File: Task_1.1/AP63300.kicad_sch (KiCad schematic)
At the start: 10 parts, among them J1 Conn_01x03, U1 AP63300

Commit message: Fixed and updated part numbers and pcb schematics
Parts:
- C1: footprint Capacitor_SMD:C_1206_3216Metric -> Capacitor_SMD:C_1210_3225Metric
- C21, C22: footprint Capacitor_SMD:C_0201_0603Metric -> Capacitor_SMD:C_1210_3225Metric
- C3: footprint Capacitor_SMD:C_0201_0603Metric -> Capacitor_SMD:C_0603_1608Metric; MPN GRM033C71C104KE14D -> CC0603KRX7R7BB104
- C4: footprint Capacitor_SMD:C_0201_0603Metric -> Capacitor_SMD:C_0603_1608Metric; MPN GRM0335C1E470FA01D -> 885012006021
- R1: footprint Resistor_SMD:R_0201_0603Metric -> Resistor_SMD:R_0603_1608Metric; MPN ERJ-1GNF1583C -> RC0603FR-07158KL
- R2: footprint Resistor_SMD:R_0201_0603Metric -> Resistor_SMD:R_0603_1608Metric; MPN ERJ-1GNF3012C -> RK73H1JTTD3012F
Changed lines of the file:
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@@
 			)
 		)
-		(property "Footprint" "Resistor_SMD:R_0201_0603Metric"
+		(property "Footprint" "Resistor_SMD:R_0603_1608Metric"
 			(at 99.822 59.69 90)
 			(hide yes)
@@
 			)
 		)
-		(property "Datasheet" "https://industrial.panasonic.com/cdbs/www-data/pdf/RDA0000/AOA0000C304.pdf"
+		(property "Datasheet" "https://www.koaspeer.com/pdfs/RK73H.pdf"
 			(at 101.6 59.69 0)
 			(hide yes)
@@
 			)
 		)
-		(property "Description" "30.1 kOhms ±1% 0.05W, 1/20W Chip Resistor 0201 (0603 Metric) Thick Film"
+		(property "Description" "30.1 kOhms ±1% 0.1W, 1/10W Chip Resistor 0603 (1608 Metric) Automotive AEC-Q200 Thick Film"
 			(at 101.6 59.69 0)
 			(hide yes)
@@
 			)
 		)
-		(property "MPN" "ERJ-1GNF3012C"
+		(property "MPN" "RK73H1JTTD3012F"
 			(at 101.6 59.69 0)
 			(hide yes)
@@
 			)
 		)
-		(property "Footprint" "Capacitor_SMD:C_0201_0603Metric"
+		(property "Footprint" "Capacitor_SMD:C_1210_3225Metric"
 			(at 120.3452 59.69 0)
 			(hide yes)
@@
 			)
 		)
-		(property "Footprint" "Resistor_SMD:R_0201_0603Metric"
+		(property "Footprint" "Resistor_SMD:R_0603_1608Metric"
 			(at 99.822 52.07 90)
 			(hide yes)
@@
 			)
 		)
-		(property "Datasheet" "https://industrial.panasonic.com/cdbs/www-data/pdf/RDA0000/AOA0000C304.pdf"
+		(property "Datasheet" "https://yageogroup.com/content/datasheet/asset/file/PYU-RC_GROUP_51_ROHS_L"
 			(at 101.6 52.07 0)
 			(hide yes)
@@
 			)
 		)
-		(property "Description" "158 kOhms ±1% 0.05W, 1/20W Chip Resistor 0201 (0603 Metric) Thick Film"
+		(property "Description" "158 kOhms ±1% 0.1W, 1/10W Chip Resistor 0603 (1608 Metric) Moisture Resistant Thick Film"
 			(at 101.6 52.07 0)
 			(hide yes)
@@
 			)
 		)
-		(property "MPN" "ERJ-1GNF1583C"
+		(property "MPN" "RC0603FR-07158KL"
 			(at 101.6 52.07 0)
 			(hide yes)
@@
 			)
 		)
-		(property "Footprint" "Capacitor_SMD:C_0201_0603Metric"
+		(property "Footprint" "Capacitor_SMD:C_0603_1608Metric"
 			(at 96.2152 55.88 0)
 			(hide yes)
@@
 			)
 		)
-		(property "Datasheet" "https://mm.digikey.com/Volume0/opasdata/d220001/medias/docus/8942/490_Chip_Multilayer_CAT2021_MLCC.pdf"
+		(property "Datasheet" "https://www.we-online.com/components/products/datasheet/885012006021.pdf"
 			(at 95.25 52.07 0)
 			(hide yes)
@@
 			)
 		)
-		(property "Description" "47 pF ±1% 25V Ceramic Capacitor C0G, NP0 0201 (0603 Metric)"
+		(property "Description" "47 pF ±5% 16V Ceramic Capacitor C0G, NP0 0603 (1608 Metric)"
 			(at 95.25 52.07 0)
 			(hide yes)
@@
 			)
 		)
-		(property "MPN" "GRM0335C1E470FA01D"
+		(property "MPN" "885012006021"
 			(at 95.25 52.07 0)
 			(hide yes)
@@
 			)
 		)
-		(property "Footprint" "Capacitor_SMD:C_1206_3216Metric"
+		(property "Footprint" "Capacitor_SMD:C_1210_3225Metric"
 			(at 39.0652 57.15 0)
 			(hide yes)
@@
 			)
 		)
-		(property "Footprint" "Capacitor_SMD:C_0201_0603Metric"
+		(property "Footprint" "Capacitor_SMD:C_0603_1608Metric"
 			(at 83.82 49.8348 0)
 			(hide yes)
@@
 			)
 		)
-		(property "Datasheet" "https://mm.digikey.com/Volume0/opasdata/d220001/medias/docus/8942/490_Chip_Multilayer_CAT2021_MLCC.pdf"
+		(property "Datasheet" "https://yageogroup.com/content/datasheet/asset/file/UPY-GPHC_X7R_6_3V-TO-250V"
 			(at 80.01 50.8 0)
 			(hide yes)
@@
 			)
 		)
-		(property "Description" "0.1 µF ±10% 16V Ceramic Capacitor X7S 0201 (0603 Metric)"
+		(property "Description" "0.1 µF ±10% 16V Ceramic Capacitor X7R 0603 (1608 Metric)"
 			(at 80.01 50.8 0)
 			(hide yes)
@@
 			)
 		)
-		(property "MPN" "GRM033C71C104KE14D"
+		(property "MPN" "CC0603KRX7R7BB104"
 			(at 80.01 50.8 90)
 			(hide yes)
@@
 			)
 		)
-		(property "Footprint" "Capacitor_SMD:C_0201_0603Metric"
+		(property "Footprint" "Capacitor_SMD:C_1210_3225Metric"
 			(at 113.9952 59.69 0)
 			(hide yes)

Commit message: Added U1, J1 part numbers; added copper pour and vias to GND, added 3d model for L1
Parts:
- J1: MPN (none) -> PH1-03-UA
- U1: MPN (none) -> AP63300WU-7
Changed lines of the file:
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@@
+			)
+		)
+		(property "MPN" "AP63300WU-7"
+			(at 64.77 50.8 0)
+			(hide yes)
+			(show_name no)
+			(do_not_autoplace no)
+			(effects
+				(font
+					(size 1.27 1.27)
+				)
 			)
 		)
@@
 			)
 		)
-		(property "Datasheet" ""
+		(property "Datasheet" "https://app.adam-tech.com/products/download/data_sheet/201605/ph1-xx-ua-data-sheet.pdf"
 			(at 33.02 33.02 0)
 			(hide yes)
@@
 			)
 		)
-		(property "Description" "Generic connector, single row, 01x03, script generated (kicad-library-utils/schlib/autogen/connector/)"
+		(property "Description" "Connector Header Through Hole 3 position 0.100{dblquote} (2.54mm)"
 			(at 33.02 33.02 0)
 			(hide yes)
 			(show_name no)
+			(do_not_autoplace no)
+			(effects
+				(font
+					(size 1.27 1.27)
+				)
+			)
+		)
+		(property "MPN" "PH1-03-UA"
+			(at 33.02 33.02 90)
+			(hide yes)
+			(show_name no)

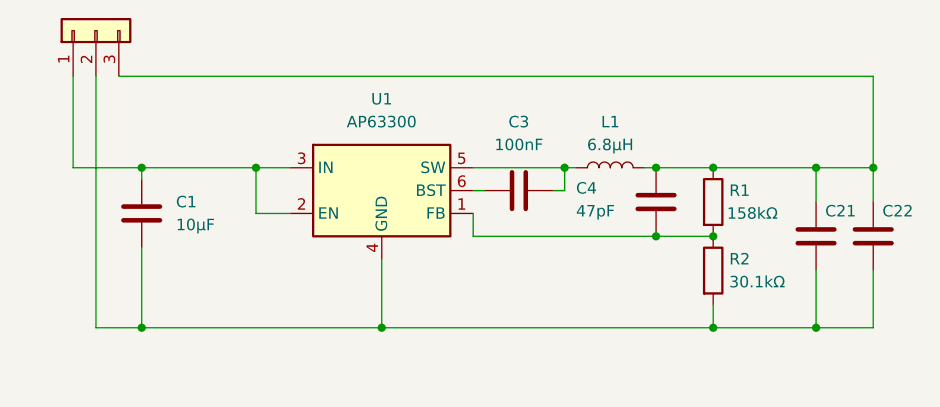
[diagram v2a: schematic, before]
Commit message: Uploaded pics for the pdf report
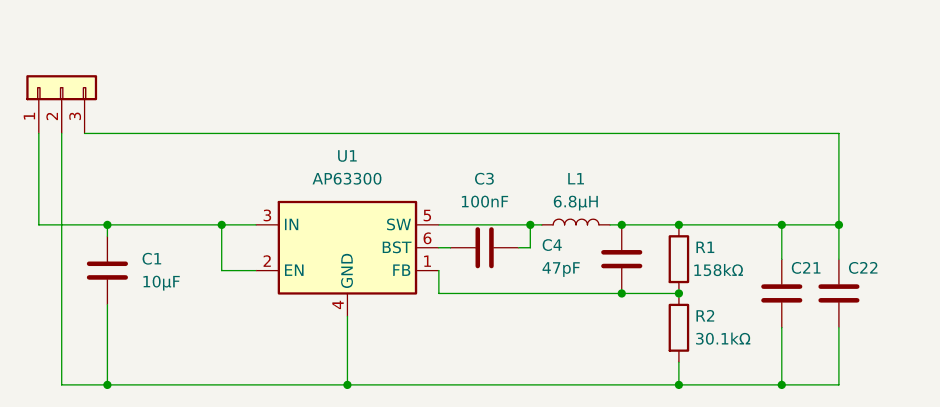
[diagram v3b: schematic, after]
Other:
- company: (none) -> AGH
- title: (none) -> AP63300 Schematic
- moved on the sheet: C1, C21, C22, C3, C4, L1, R1, R2, U1
